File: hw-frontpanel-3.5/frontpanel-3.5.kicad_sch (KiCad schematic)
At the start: 44 parts, among them J1 SPI, J2 QWIIC, J3 LED, J4 TC2030, J5 OLED_SH1107, SW1 SW_Push, SW2 SW_Push, SW3 SW_Push, SW4 SW_Push, U1 MT3540, U2 LM809, U3 ESP32-C3-MINI-1

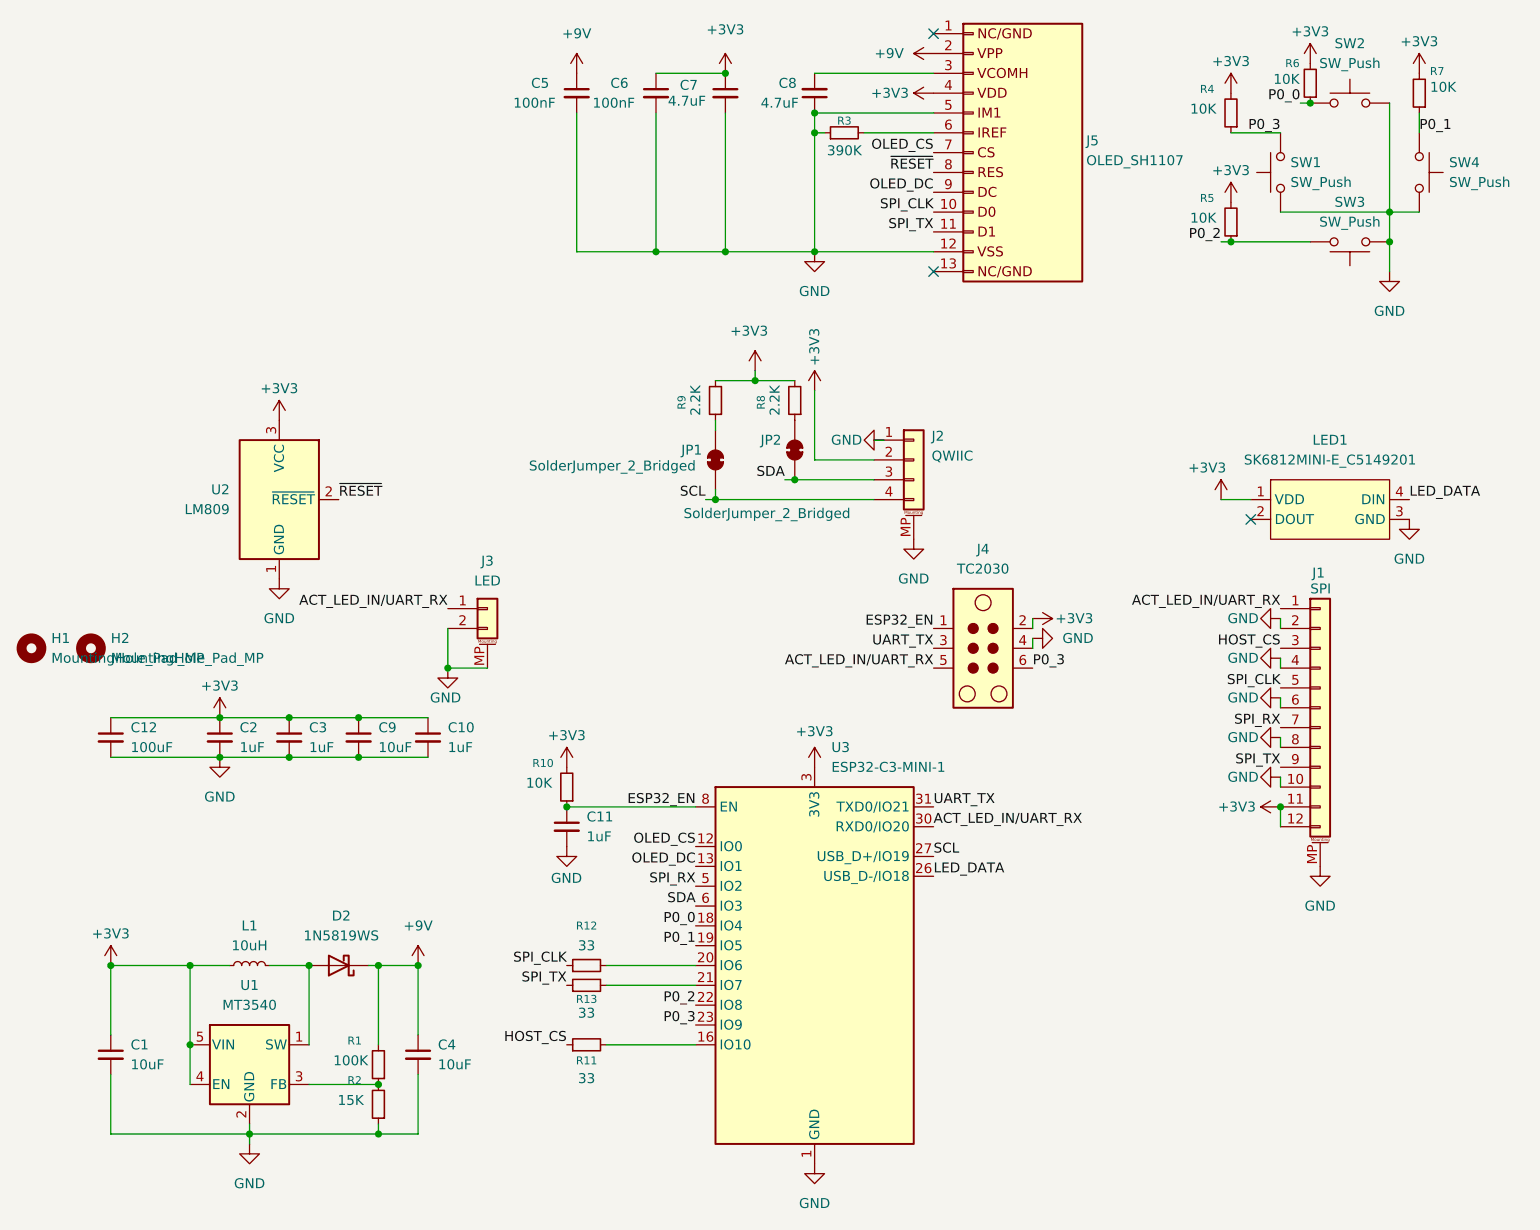
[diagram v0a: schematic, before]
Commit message: Final v1.0.0 front panel design
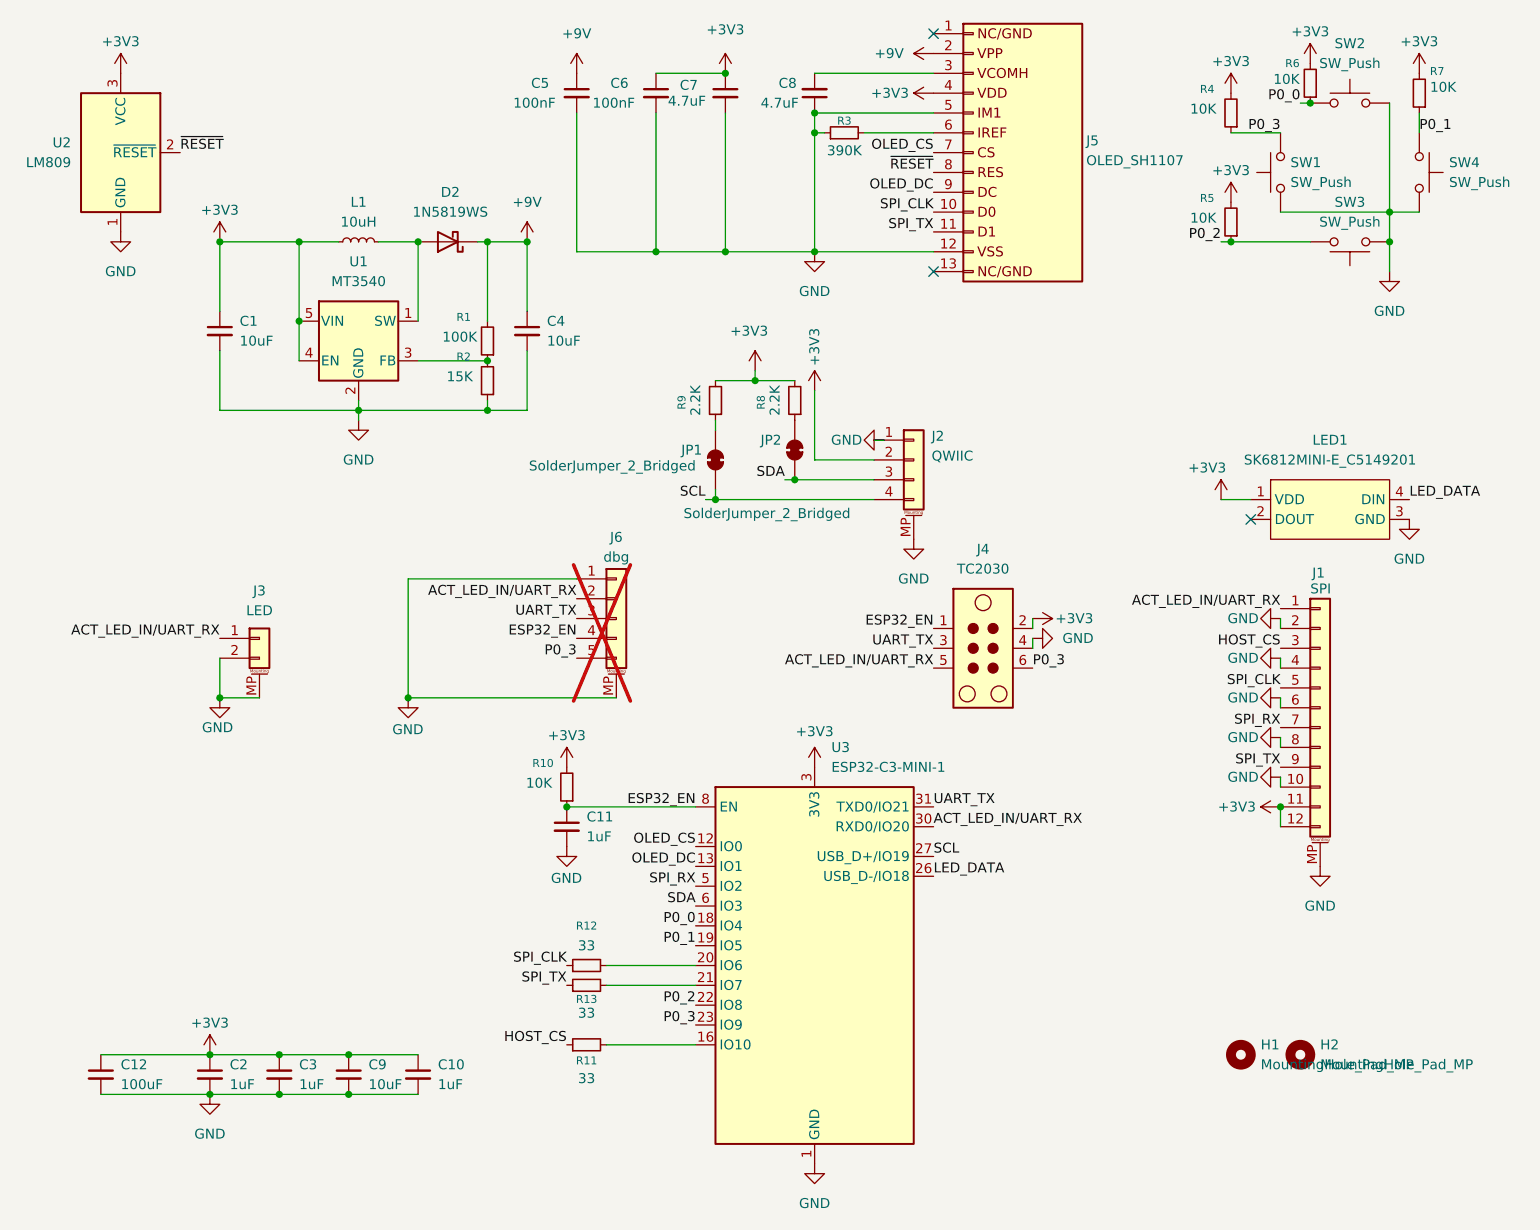
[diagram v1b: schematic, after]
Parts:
- added J6: dbg, Connector_JST:JST_SH_BM05B-SRSS-TB_1x05-1MP_P1.00mm_Vertical, symbol Connector_Generic_MountingPin:Conn_01x05_MountingPin
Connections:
- net ACT_LED_IN/UART_RX: now also J6.2 (Pin_2)
- net ESP32_EN: now also J6.4 (Pin_4)
- net GND: now also J6.1 (Pin_1), J6.MP (MountPin)
- net P0_3: now also J6.5 (Pin_5)
- net UART_TX: now also J6.3 (Pin_3)
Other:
- moved on the sheet: C1, C10, C12, C2, C3, C4, C9, D2, H1, H2, J3, L1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
